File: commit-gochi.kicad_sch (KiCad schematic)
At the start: 15 parts, among them J1 USB_C_Receptacle_USB2.0_16P, J2 Conn_01x04_Socket, Q1 Q_NPN_BCE, SW1 SW_Push, U1 ESP32-C3_SUPERMINI_TH

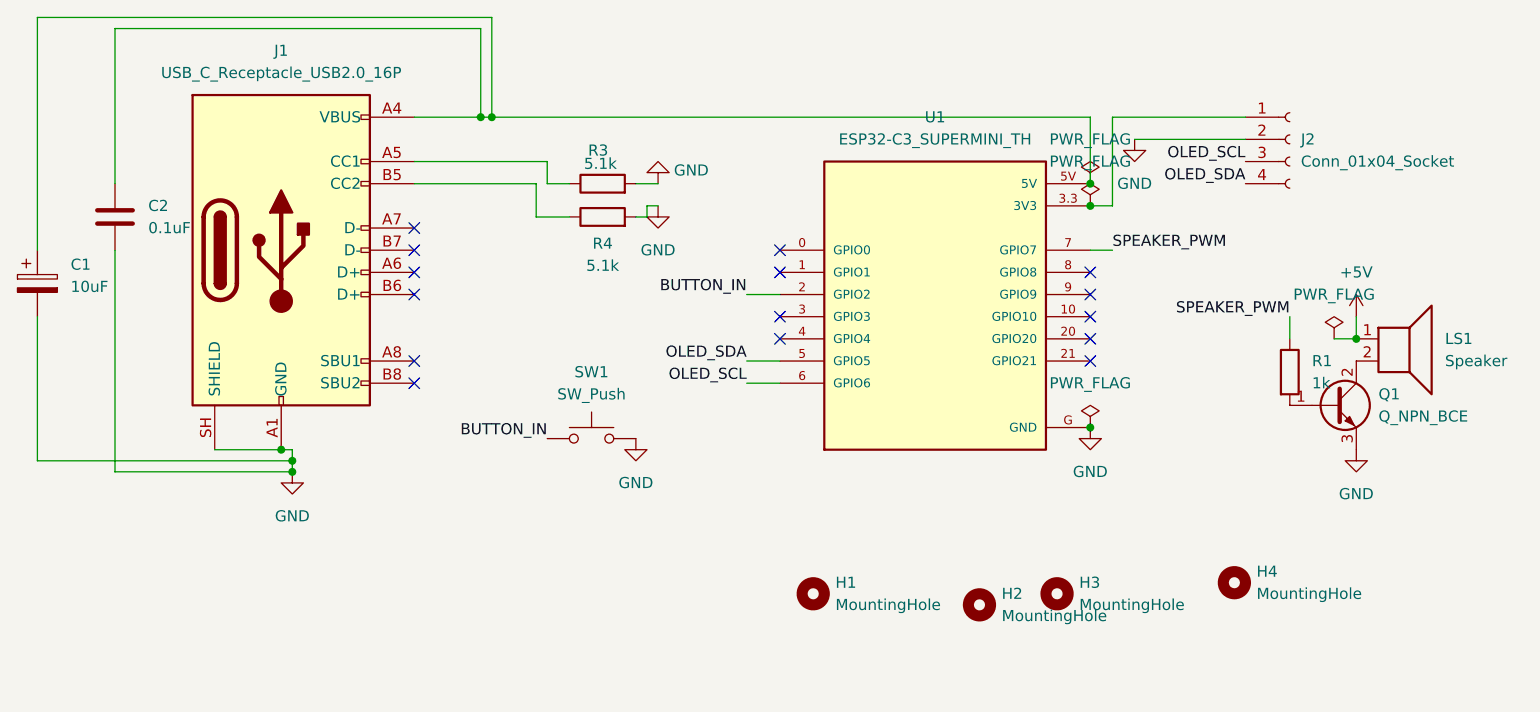
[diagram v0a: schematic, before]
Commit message: Add files via upload
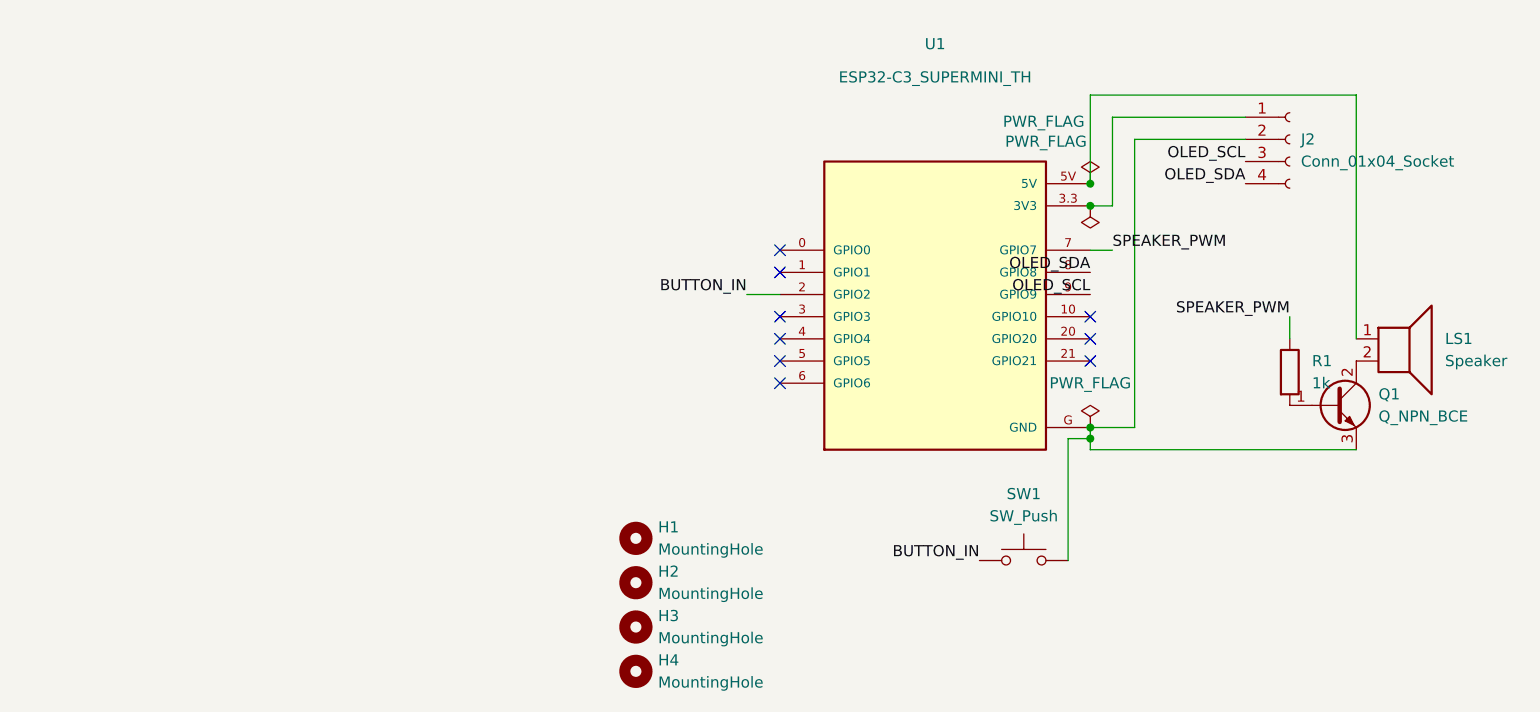
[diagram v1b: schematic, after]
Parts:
- removed C1: 10uF, Capacitor_THT:CP_Radial_D5.0mm_P2.00mm, symbol Device:C_Polarized
- removed C2: 0.1uF, Capacitor_THT:C_Disc_D3.8mm_W2.6mm_P2.50mm, symbol Device:C
- removed J1: USB_C_Receptacle_USB2.0_16P, Connector_USB:USB_C_Receptacle_HRO_TYPE-C-31-M-12, symbol Connector:USB_C_Receptacle_USB2.0_16P
- removed R3, R4: 5.1k, Resistor_THT:R_Axial_DIN0207_L6.3mm_D2.5mm_P7.62mm_Horizontal, symbol Device:R
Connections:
- net +5V is gone; now on an unnamed net: LS1.1
- net OLED_SCL: now also U1.9 (GPIO9); no longer U1.6 (GPIO6)
- net OLED_SDA: now also U1.8 (GPIO8); no longer U1.5 (GPIO5)
- net GND: no longer names the net of J2.2 (GND), Q1.3 (E), SW1.2, U1.G (GND)
- no-connect marks 15 -> 9
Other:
- moved on the sheet: H1, SW1
